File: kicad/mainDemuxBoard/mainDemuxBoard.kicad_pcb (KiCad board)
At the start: 2 copper layers, 217 parts, among them J1 Conn_02x20_Top_Bottom, J10 Conn_02x20_Top_Bottom, J11 Conn_02x20_Top_Bottom, J12 Conn_02x20_Top_Bottom, J13 Conn_02x20_Top_Bottom, J14 Conn_02x20_Top_Bottom, J15 Conn_02x20_Top_Bottom, J16 Conn_02x20_Top_Bottom, J17 Conn_02x20_Top_Bottom, J2 Conn_02x20_Top_Bottom, J3 Conn_02x20_Top_Bottom, J4 Conn_02x20_Top_Bottom, J5 Conn_02x20_Top_Bottom, J6 Conn_02x20_Top_Bottom, J7 Conn_02x20_Top_Bottom, J8 Conn_02x20_Top_Bottom, J9 Conn_02x20_Top_Bottom, Q1 PMOS, Q10 PMOS, Q100 PMOS, Q101 PMOS, Q102 PMOS, Q103 PMOS, Q104 NMOS, Q105 NMOS, Q106 NMOS, Q107 NMOS, Q108 NMOS, Q109 PMOS, Q11 PMOS, Q110 PMOS, Q111 PMOS, Q112 PMOS, Q113 PMOS, Q114 NMOS, Q115 NMOS, Q116 NMOS, Q117 NMOS, Q118 NMOS, Q119 PMOS, Q12 PMOS, Q120 PMOS, Q121 PMOS, Q122 PMOS, Q123 PMOS, Q124 NMOS, Q125 NMOS, Q126 NMOS, Q127 NMOS, Q128 NMOS, Q129 PMOS, Q13 PMOS, Q130 PMOS, Q131 PMOS, Q132 PMOS, Q133 PMOS, Q134 NMOS, Q135 NMOS, Q136 NMOS, Q137 NMOS, Q138 NMOS, Q139 PMOS, Q14 NMOS, Q140 PMOS, Q141 PMOS, Q142 PMOS, Q143 PMOS, Q144 NMOS, Q145 NMOS, Q146 NMOS, Q147 NMOS, Q148 NMOS, Q149 PMOS, Q15 NMOS, Q150 PMOS, Q151 PMOS, Q152 PMOS, Q153 PMOS, Q154 NMOS, Q155 NMOS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

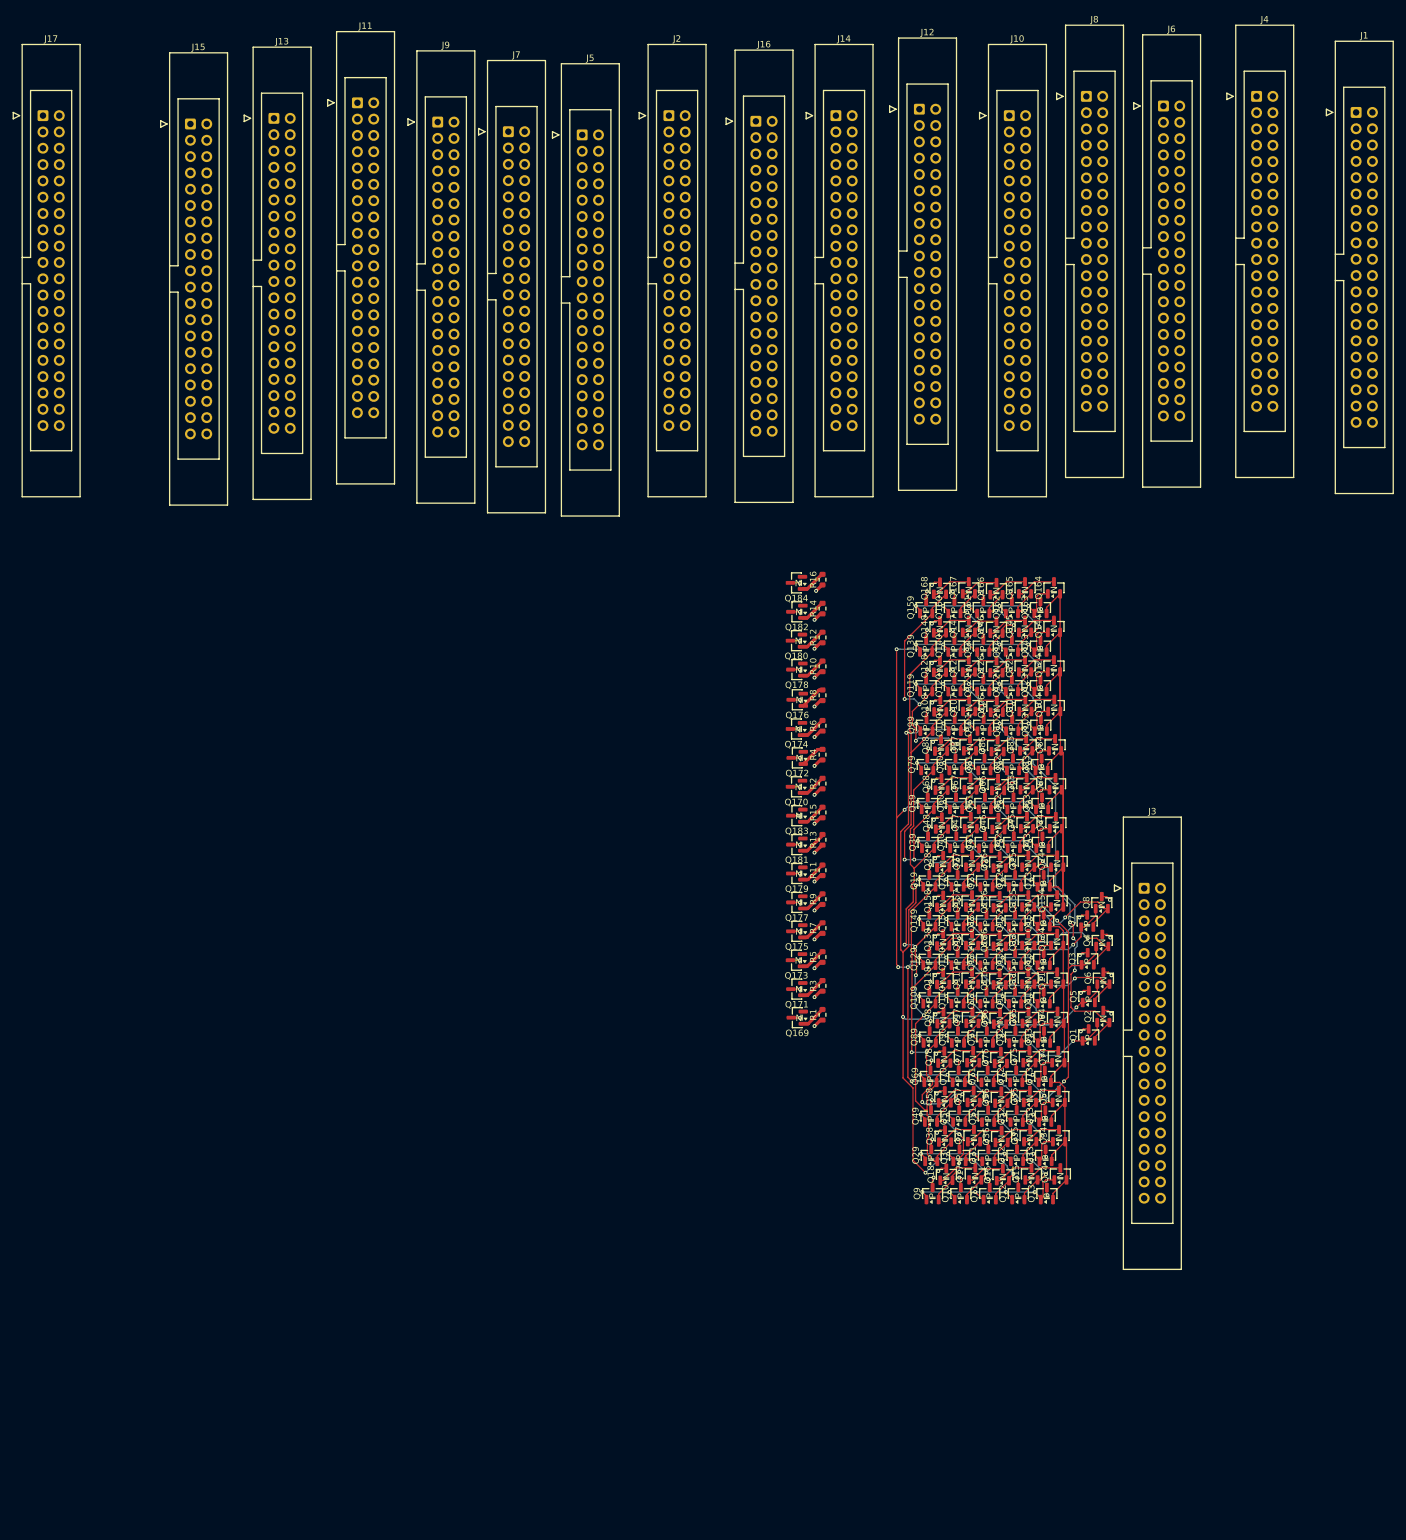
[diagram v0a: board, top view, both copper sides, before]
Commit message: finish main demux board
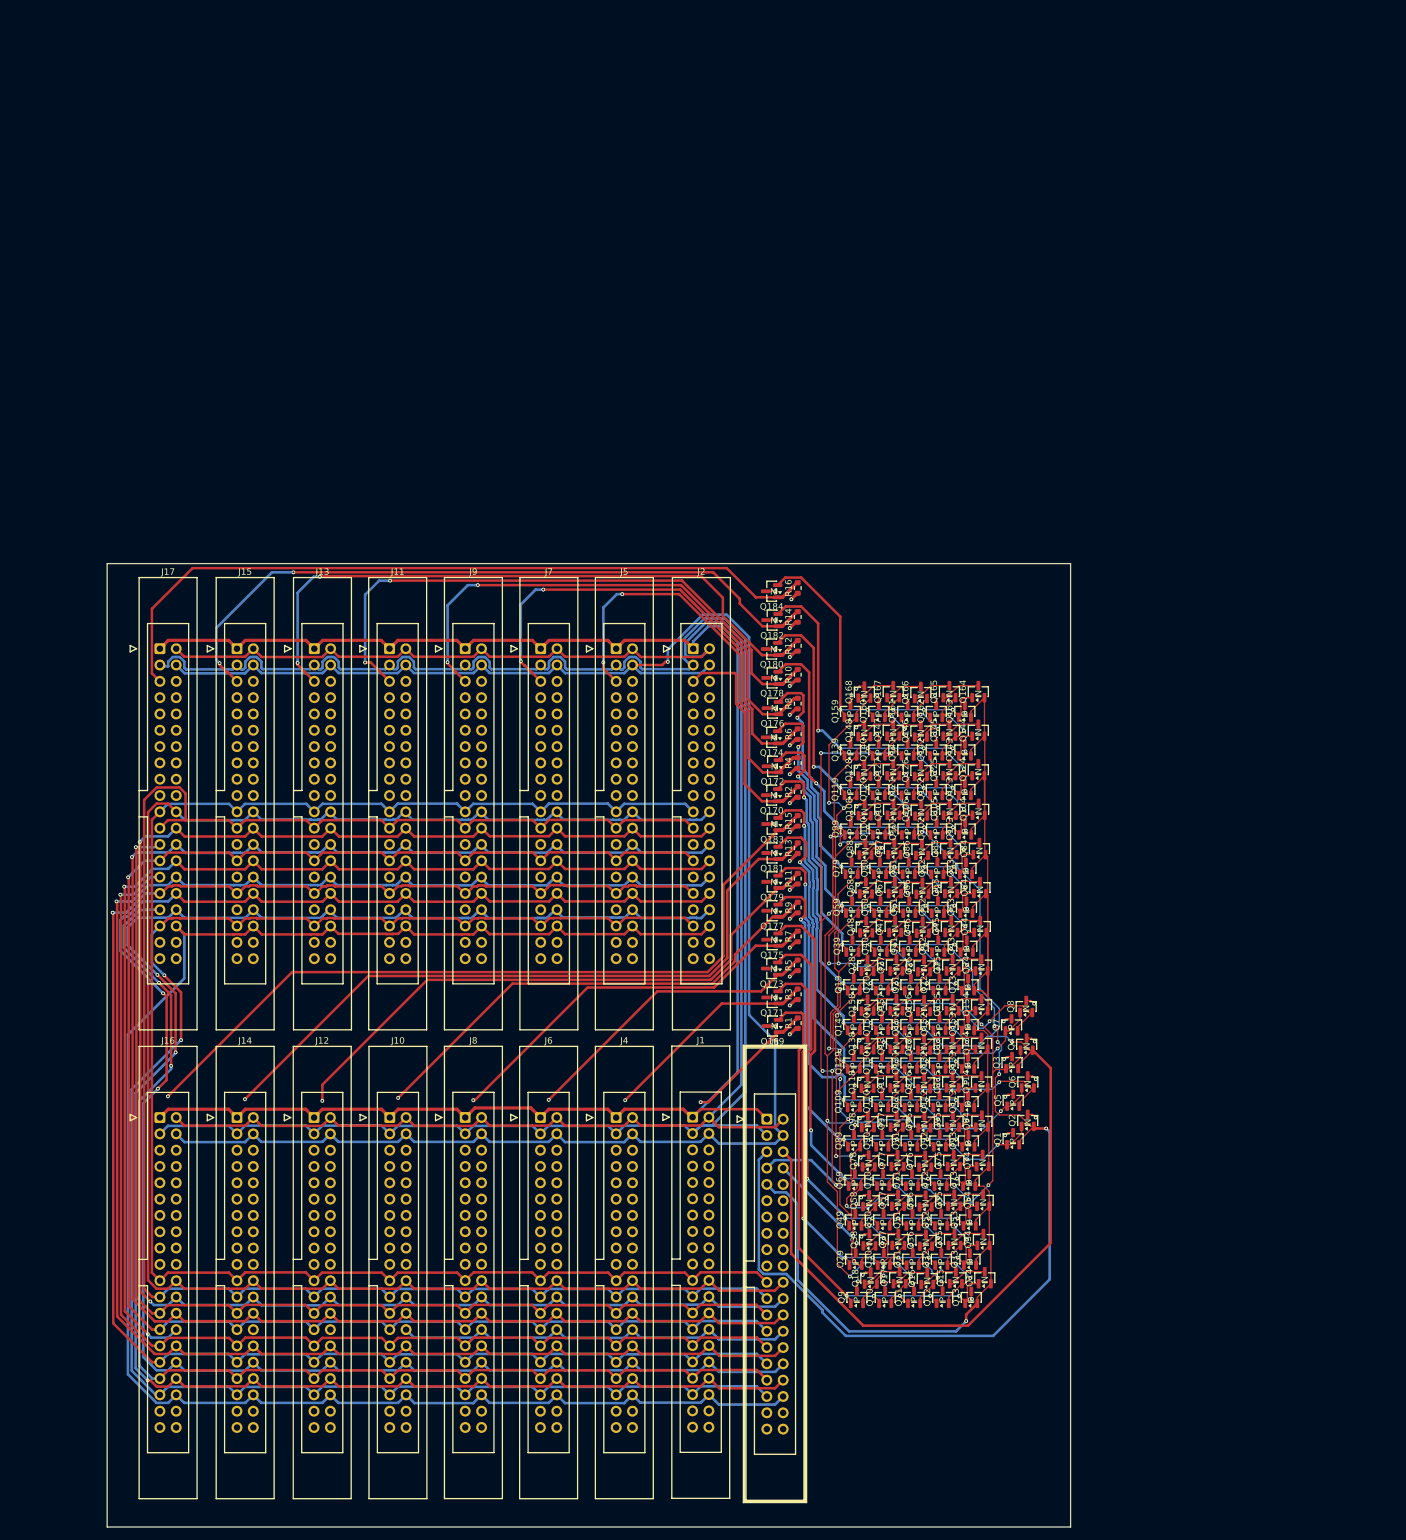
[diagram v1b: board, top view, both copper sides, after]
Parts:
- moved J4 187.7 mm to (109.2, 105.0)
- moved J1 187.5 mm to (121.2, 105.0)
- moved J8 186.1 mm to (85.8, 105.0)
- moved J6 185.0 mm to (97.5, 105.0)
- moved J10 183.4 mm to (74.0, 105.0)
- moved J12 183.1 mm to (62.2, 105.0)
- moved J14 181.7 mm to (50.2, 105.0)
- moved J16 180.8 mm to (38.2, 105.0)
- moved J11 85.1 mm to (74.0, 32.0)
- moved J17 85.0 mm to (38.2, 32.0)
- moved J2 83.1 mm to (121.2, 32.0)
- moved J13 82.8 mm to (62.2, 32.0)
- moved J9 82.1 mm to (85.8, 32.0)
- moved J15 82.0 mm to (50.2, 32.0)
- moved J7 80.7 mm to (97.5, 32.0)
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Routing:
- net /S_{2}: track 0.00 -> 306.9 mm
- net /S_{3}: track 0.00 -> 297.1 mm, vias 0 -> 1
- net /S_{1}: track 0.00 -> 287.2 mm
- net /~{BL_{6}}: track 0.00 -> 284.4 mm, vias 0 -> 3
- net /BL_{1}: track 0.00 -> 284.2 mm
- net /~{BL_{5}}: track 0.00 -> 283.0 mm, vias 0 -> 2
- net /S_{0}: track 0.00 -> 281.1 mm
- net /~{BL_{4}}: track 0.00 -> 281.1 mm, vias 0 -> 1
- net /~{BL_{2}}: track 0.00 -> 278.9 mm, vias 0 -> 1
- net /~{BL_{0}}: track 0.00 -> 277.4 mm
- net /~{BL_{7}}: track 0.00 -> 277.2 mm
- net /~{BL_{1}}: track 0.00 -> 276.9 mm, vias 0 -> 2
- net /BL_{5}: track 0.00 -> 276.6 mm, vias 0 -> 1
- net /BL_{7}: track 0.00 -> 274.5 mm, vias 0 -> 2
- net /BL_{3}: track 0.00 -> 272.5 mm, vias 0 -> 1
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- added copper zone on In2.Cu, net +10V
- added copper zone on In2.Cu, net +5V
- added copper zone on In1.Cu, net GND
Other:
- board outline added: 150 x 150 mm
- copper layers 2 -> 4
